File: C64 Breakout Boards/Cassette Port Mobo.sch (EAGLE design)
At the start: 2 parts

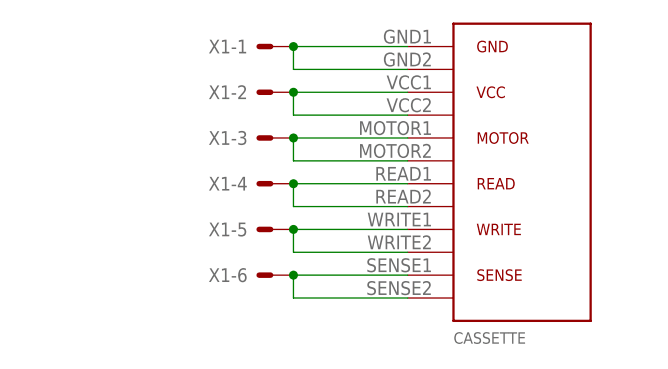
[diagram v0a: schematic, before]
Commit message: More expansion board work
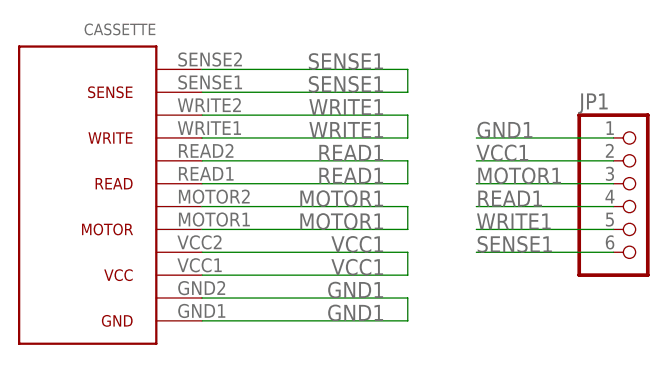
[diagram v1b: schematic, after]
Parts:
- removed X1: (no value), con-molex:22-23-2061
- added JP1: (no value), pinhead:PINHD-1X6
- CASSETTE: device myparts:C64_CASSETTE -> 0myparts:C64_CASSETTE
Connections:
- removed net N$1: CASSETTE.GND1, CASSETTE.GND2, X1-1.S
- removed net N$11: CASSETTE.SENSE1, CASSETTE.SENSE2, X1-6.S
- removed net N$3: CASSETTE.VCC1, CASSETTE.VCC2, X1-2.S
- removed net N$5: CASSETTE.MOTOR1, CASSETTE.MOTOR2, X1-3.S
- removed net N$7: CASSETTE.READ1, CASSETTE.READ2, X1-4.S
- removed net N$9: CASSETTE.WRITE1, CASSETTE.WRITE2, X1-5.S
- new net GND1: CASSETTE.GND1, CASSETTE.GND2, JP1.1
- new net MOTOR1: CASSETTE.MOTOR1, CASSETTE.MOTOR2, JP1.3
- new net READ1: CASSETTE.READ1, CASSETTE.READ2, JP1.4
- new net SENSE1: CASSETTE.SENSE1, CASSETTE.SENSE2, JP1.6
- new net VCC1: CASSETTE.VCC1, CASSETTE.VCC2, JP1.2
- new net WRITE1: CASSETTE.WRITE1, CASSETTE.WRITE2, JP1.5
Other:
- moved on the sheet: CASSETTE
